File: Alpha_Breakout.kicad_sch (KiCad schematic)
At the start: 0 parts

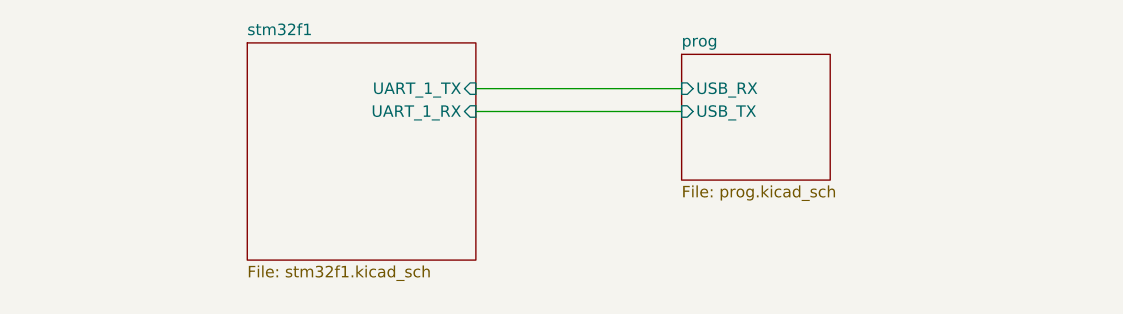
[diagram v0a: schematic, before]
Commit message: adcs
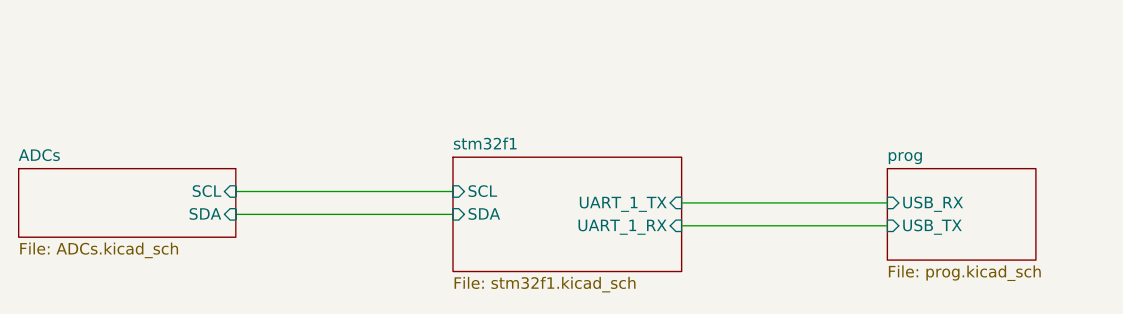
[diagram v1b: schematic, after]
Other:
- added sheet ADCs (ADCs.kicad_sch)
- sheet stm32f1 ports: added SCL, SDA; removed none
- title: (none) -> Alpha_Peripheral_Board
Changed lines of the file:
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@@
 	(generator_version "9.0")
 	(paper "A4")
-	(wire
-		(pts
-			(xy 143.51 83.82) (xy 166.37 83.82)
-		)
-		(stroke
-			(width 0)
-			(type default)
-		)
-	)
-	(wire
-		(pts
-			(xy 143.51 81.28) (xy 166.37 81.28)
+	(title_block
+		(title "Alpha_Peripheral_Board")
+	)
+	(wire
+		(pts
+			(xy 116.84 92.71) (xy 140.97 92.71)
+		)
+		(stroke
+			(width 0)
+			(type default)
+		)
+	)
+	(wire
+		(pts
+			(xy 166.37 96.52) (xy 189.23 96.52)
+		)
+		(stroke
+			(width 0)
+			(type default)
+		)
+	)
+	(wire
+		(pts
+			(xy 166.37 93.98) (xy 189.23 93.98)
+		)
+		(stroke
+			(width 0)
+			(type default)
+		)
+	)
+	(wire
+		(pts
+			(xy 116.84 95.25) (xy 140.97 95.25)
 		)
 		(stroke
@@
 	)
 	(sheet
-		(at 118.11 76.2)
-		(size 25.4 24.13)
+		(at 140.97 88.9)
+		(size 25.4 12.7)
 		(exclude_from_sim no)
 		(in_bom yes)
@@
 		)
 		(property "Sheetname" "stm32f1"
-			(at 118.11 75.4884 0)
+			(at 140.97 88.1884 0)
 			(effects
 				(font
@@
 		)
 		(property "Sheetfile" "stm32f1.kicad_sch"
-			(at 118.11 100.9146 0)
+			(at 140.97 102.1846 0)
 			(effects
 				(font
@@
 		)
 		(pin "UART_1_TX" input
-			(at 143.51 81.28 0)
+			(at 166.37 93.98 0)
 			(effects
 				(font
@@
 		)
 		(pin "UART_1_RX" input
-			(at 143.51 83.82 0)
-			(effects
-				(font
-					(size 1.27 1.27)
-				)
-				(justify right)
+			(at 166.37 96.52 0)
+			(effects
+				(font
+					(size 1.27 1.27)
+				)
+				(justify right)
+			)
+		)
+		(pin "SDA" input
+			(at 140.97 95.25 180)
+			(effects
+				(font
+					(size 1.27 1.27)
+				)
+				(justify left)
+			)
+		)
+		(pin "SCL" input
+			(at 140.97 92.71 180)
+			(effects
+				(font
+					(size 1.27 1.27)
+				)
+				(justify left)
 			)
 		)
@@
 	)
 	(sheet
-		(at 166.37 77.47)
-		(size 16.51 13.97)
+		(at 92.71 90.17)
+		(size 24.13 7.62)
 		(exclude_from_sim no)
 		(in_bom yes)
@@
 			(color 0 0 0 0.0000)
 		)
+		(property "Sheetname" "ADCs"
+			(at 92.71 89.4584 0)
+			(effects
+				(font
+					(size 1.27 1.27)
+				)
+				(justify left bottom)
+			)
+		)
+		(property "Sheetfile" "ADCs.kicad_sch"
+			(at 92.71 98.3746 0)
+			(effects
+				(font
+					(size 1.27 1.27)
+				)
+				(justify left top)
+			)
+		)
+		(pin "SCL" input
+			(at 116.84 92.71 0)
+			(effects
+				(font
+					(size 1.27 1.27)
+				)
+				(justify right)
+			)
+		)
+		(pin "SDA" input
+			(at 116.84 95.25 0)
+			(effects
+				(font
+					(size 1.27 1.27)
+				)
+				(justify right)
+			)
+		)
+		(instances
+			(project "Alpha_Breakout"
+				(path "/bb73515c-a1ce-4448-8899-3a433fb04c26"
+					(page "4")
+				)
+			)
+		)
+	)
+	(sheet
+		(at 189.23 90.17)
+		(size 16.51 10.16)
+		(exclude_from_sim no)
+		(in_bom yes)
+		(on_board yes)
+		(dnp no)
+		(fields_autoplaced yes)
+		(stroke
+			(width 0.1524)
+			(type solid)
+		)
+		(fill
+			(color 0 0 0 0.0000)
+		)
 		(property "Sheetname" "prog"
-			(at 166.37 76.7584 0)
+			(at 189.23 89.4584 0)
 			(effects
 				(font
@@
 		)
 		(property "Sheetfile" "prog.kicad_sch"
-			(at 166.37 92.0246 0)
+			(at 189.23 100.9146 0)
 			(effects
 				(font
@@
 		)
 		(pin "USB_RX" input
-			(at 166.37 81.28 180)
+			(at 189.23 93.98 180)
 			(effects
 				(font
@@
 		)
 		(pin "USB_TX" input
-			(at 166.37 83.82 180)
-			(effects
-				(font
+			(at 189.23 96.52 180)
+			(effects
+				(font
